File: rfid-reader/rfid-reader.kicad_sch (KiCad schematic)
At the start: 16 parts, among them U1 ATmega1284-P, U2 keypad, U3 Interface_RFID_SPI, U4 LM3940I3-3.3

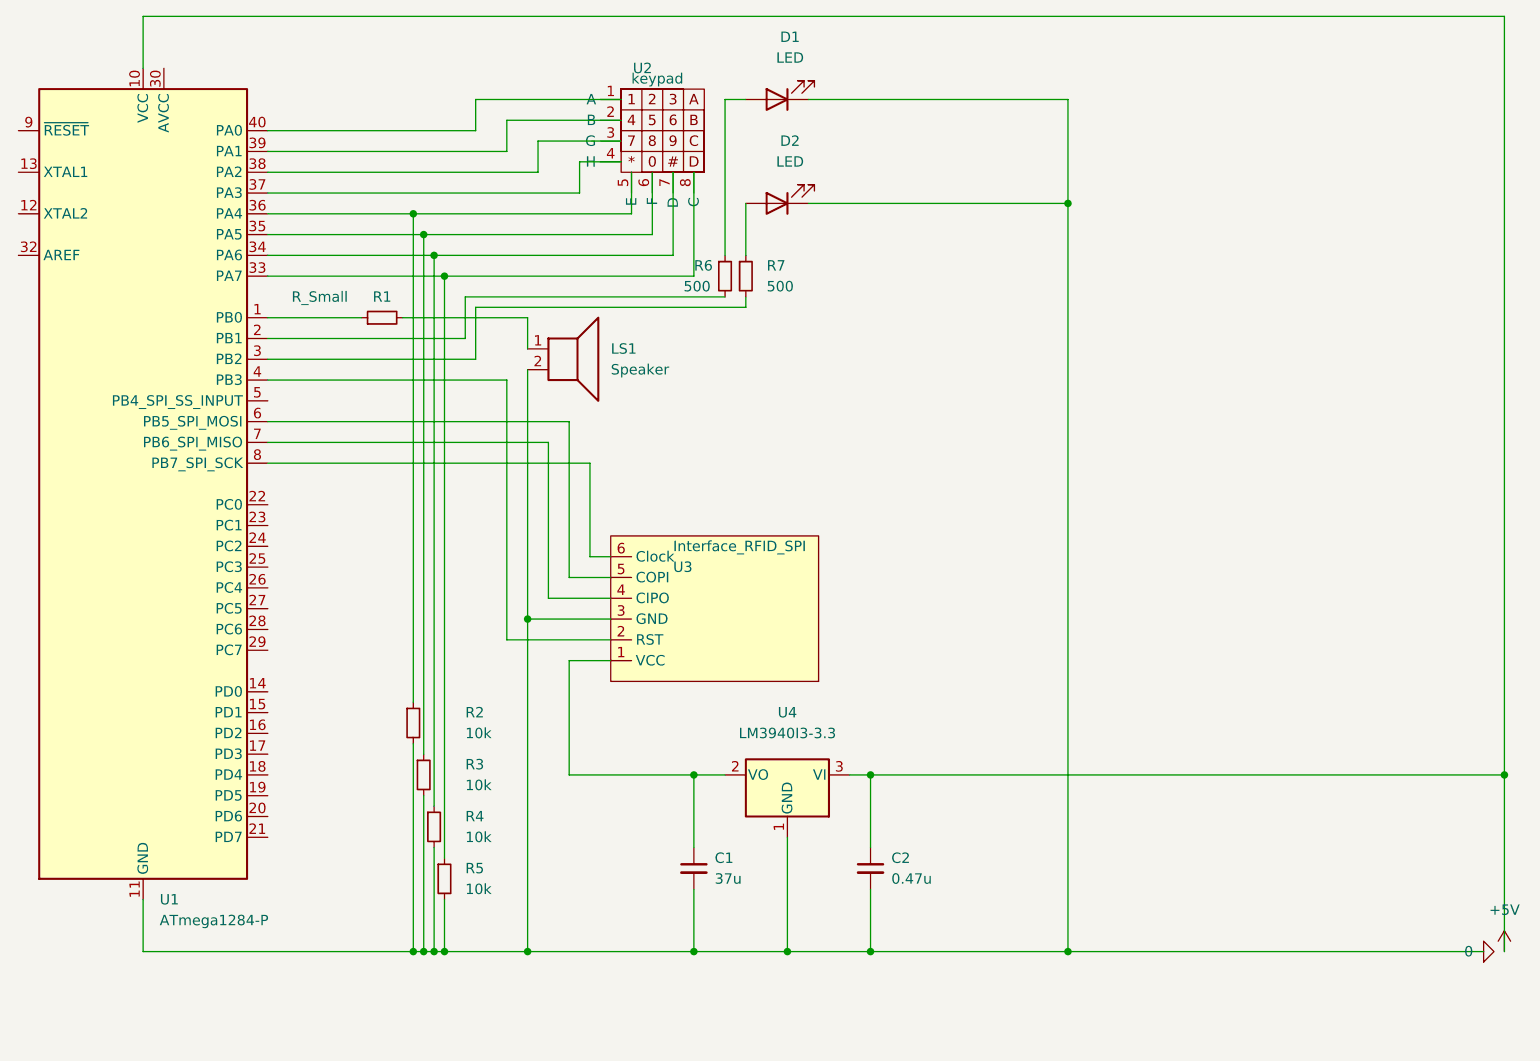
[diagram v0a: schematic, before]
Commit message: Updated schematics
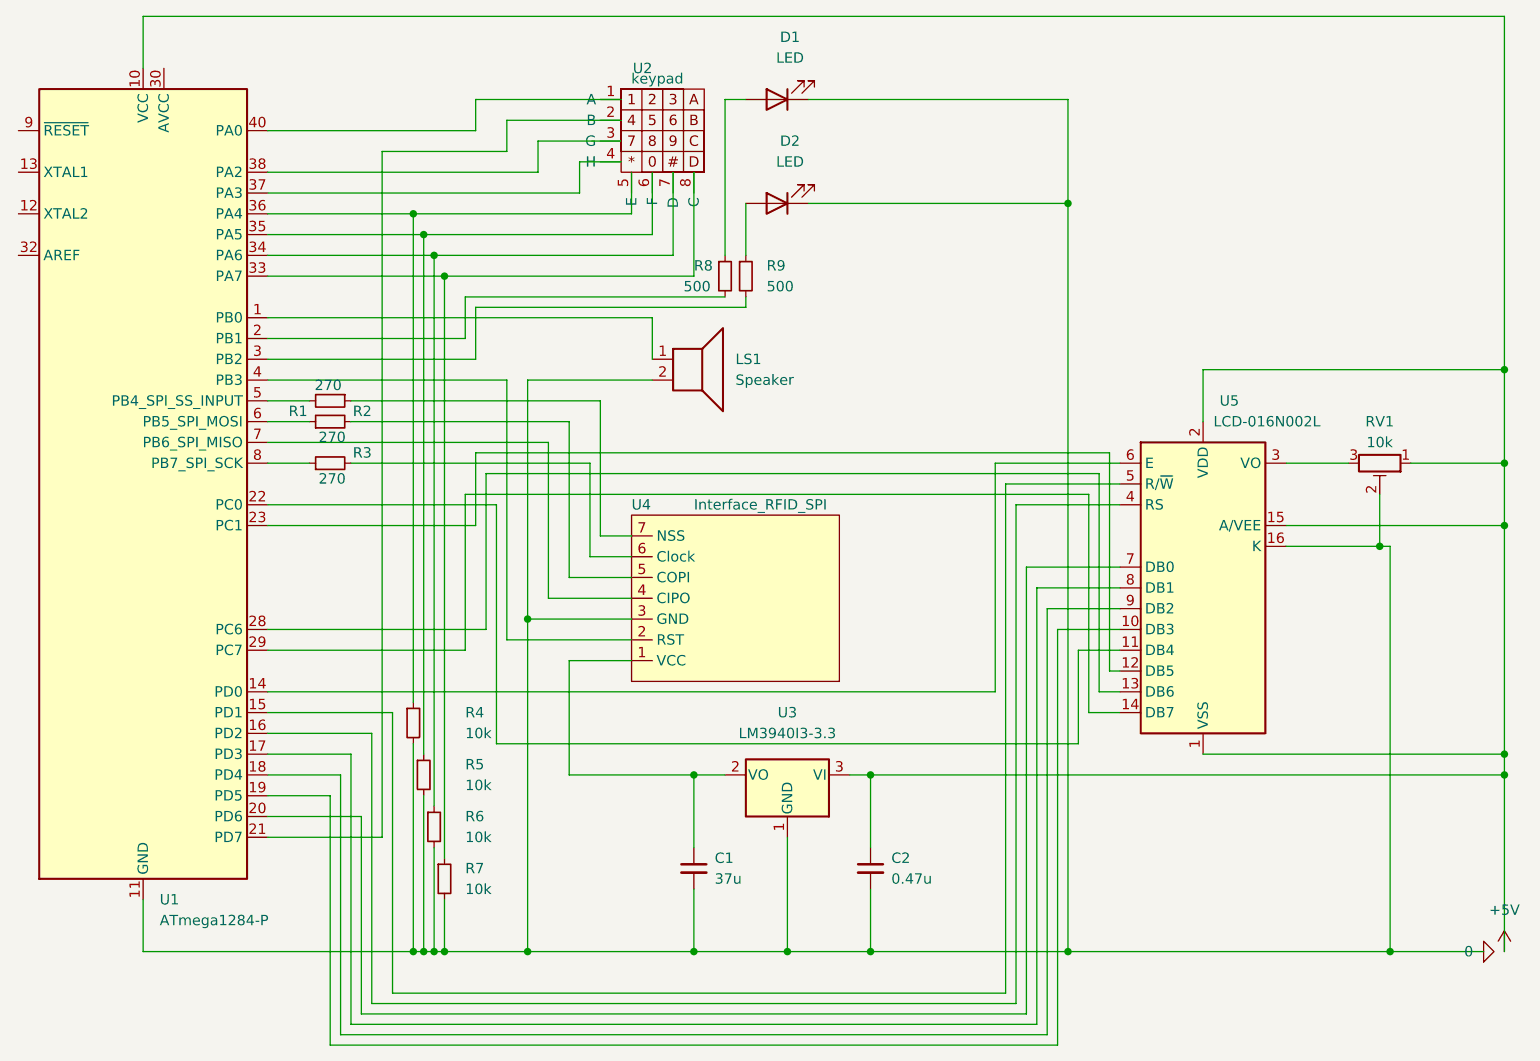
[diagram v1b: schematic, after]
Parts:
- added R2, R3: 270, symbol Device:R_Small
- added RV1: 10k, symbol Device:R_Potentiometer_Trim
- added U5: LCD-016N002L, Display:LCD-016N002L, symbol Display_Character:LCD-016N002L
- R1: value R_Small -> 270; Spice_Model (none) -> 10k; Spice_Netlist_Enabled (none) -> Y; Spice_Primitive (none) -> R
- renumbered R2 to R4, R3 to R5, R4 to R6, R5 to R7, R6 to R8, R7 to R9, U4 to U3, U3 to U4
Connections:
- net +5V: now also RV1.1, U5.1 (VSS), U5.15 (A/VEE), U5.2 (VDD)
- net 0: now also RV1.2, U5.16 (K)
- net at U2.2 (B): now also U1.21 (PD7); no longer U1.39 (PA1)
- net at U4.5 (COPI): now also R2.2; no longer U1.6 (PB5_SPI_MOSI)
- net at U4.6 (Clock): now also R3.2; no longer U1.8 (PB7_SPI_SCK)
- net at R1.1: now also U4.7 (NSS); no longer U1.1 (PB0)
- net at U1.14 (PD0): now also U5.6 (E)
- net at U1.15 (PD1): now also U5.5 (R/~{W})
- net at U1.16 (PD2): now also U5.4 (RS)
- net at U1.17 (PD3): now also U5.8 (DB1)
- net at U1.18 (PD4): now also U5.9 (DB2)
- net at U1.19 (PD5): now also U5.10 (DB3)
- net at U1.20 (PD6): now also U5.7 (DB0)
- net at U1.22 (PC0): now also U5.11 (DB4)
- net at U1.23 (PC1): now also U5.12 (DB5)
- net at U1.28 (PC6): now also U5.13 (DB6)
- net at U1.29 (PC7): now also U5.14 (DB7)
- net at U1.5 (PB4_SPI_SS_INPUT): now also R1.2
- net at LS1.1: now also U1.1 (PB0); no longer R1.2
- new net: RV1.3, U5.3 (VO)
- new net: R2.1, U1.6 (PB5_SPI_MOSI)
- new net: R3.1, U1.8 (PB7_SPI_SCK)
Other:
- moved on the sheet: LS1
